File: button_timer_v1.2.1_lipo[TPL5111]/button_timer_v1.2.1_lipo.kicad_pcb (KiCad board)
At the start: 2 copper layers, 21 x 41.7 mm, 23 parts, among them J1 Conn_01x05_Female, SW1 SW_Push, SW2 SW_Push, U2 AP2112K-3.3, U3 TPL5111, X1 ESP-12E

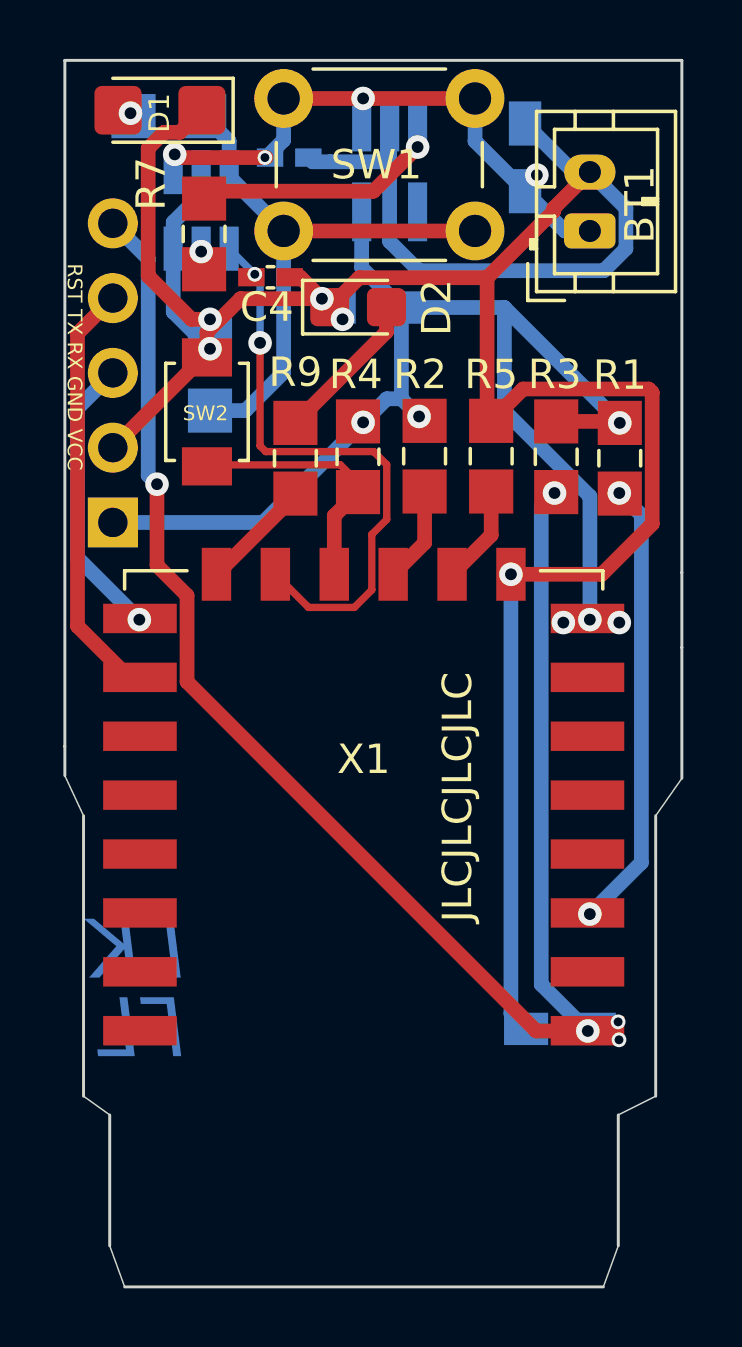
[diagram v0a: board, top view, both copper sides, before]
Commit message: Silkscreen Update
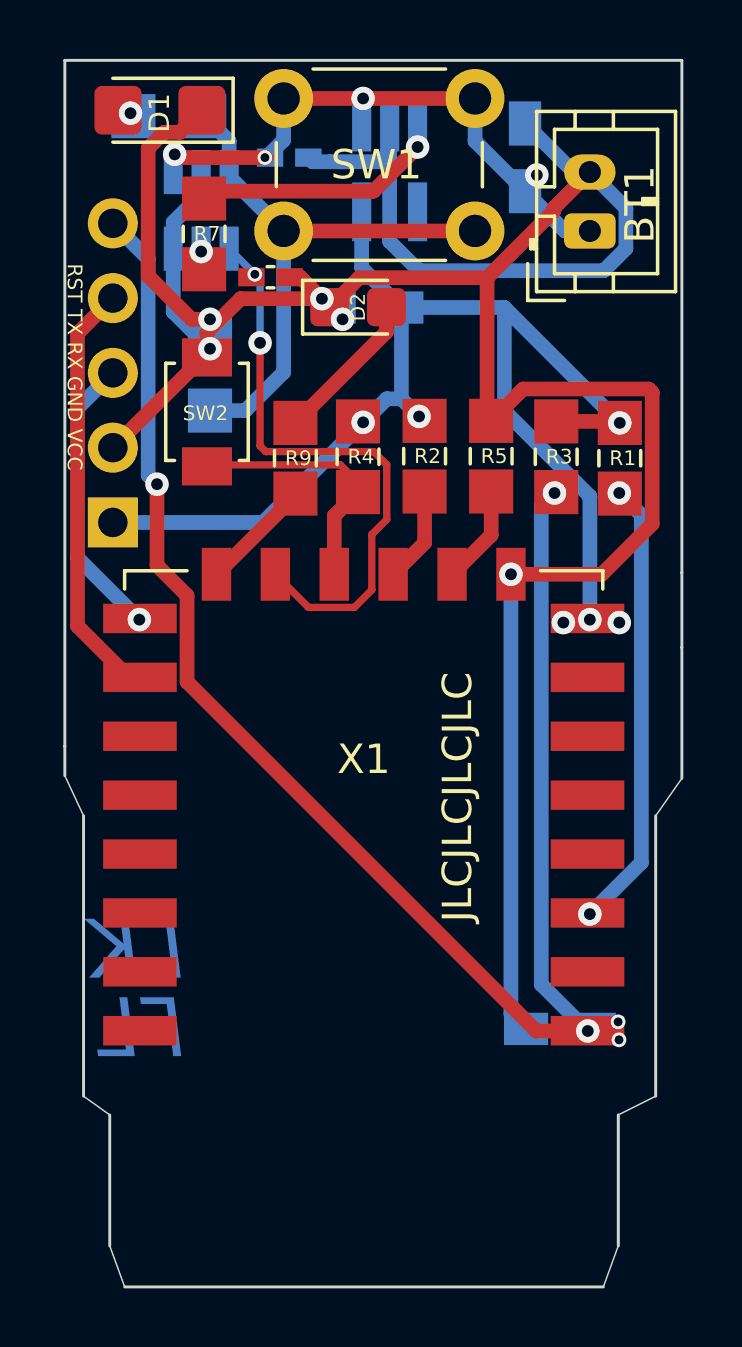
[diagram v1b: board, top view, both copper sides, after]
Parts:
- D2: footprint LED_SMD:LED_0805_2012Metric_Castellated -> handsolder:LED_0805_2012Metric_Castellated_mod
